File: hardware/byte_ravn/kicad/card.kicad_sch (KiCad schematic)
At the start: 13 parts, among them J3 Bus_Apple_II_Card_Side, U11 SN74LVC8T245, U12 SN74LVC8T245, U13 SN74LVC8T245, U14 SN74LVC8T245, U8 SN74LVC8T245, U9 SN74LVC8T245

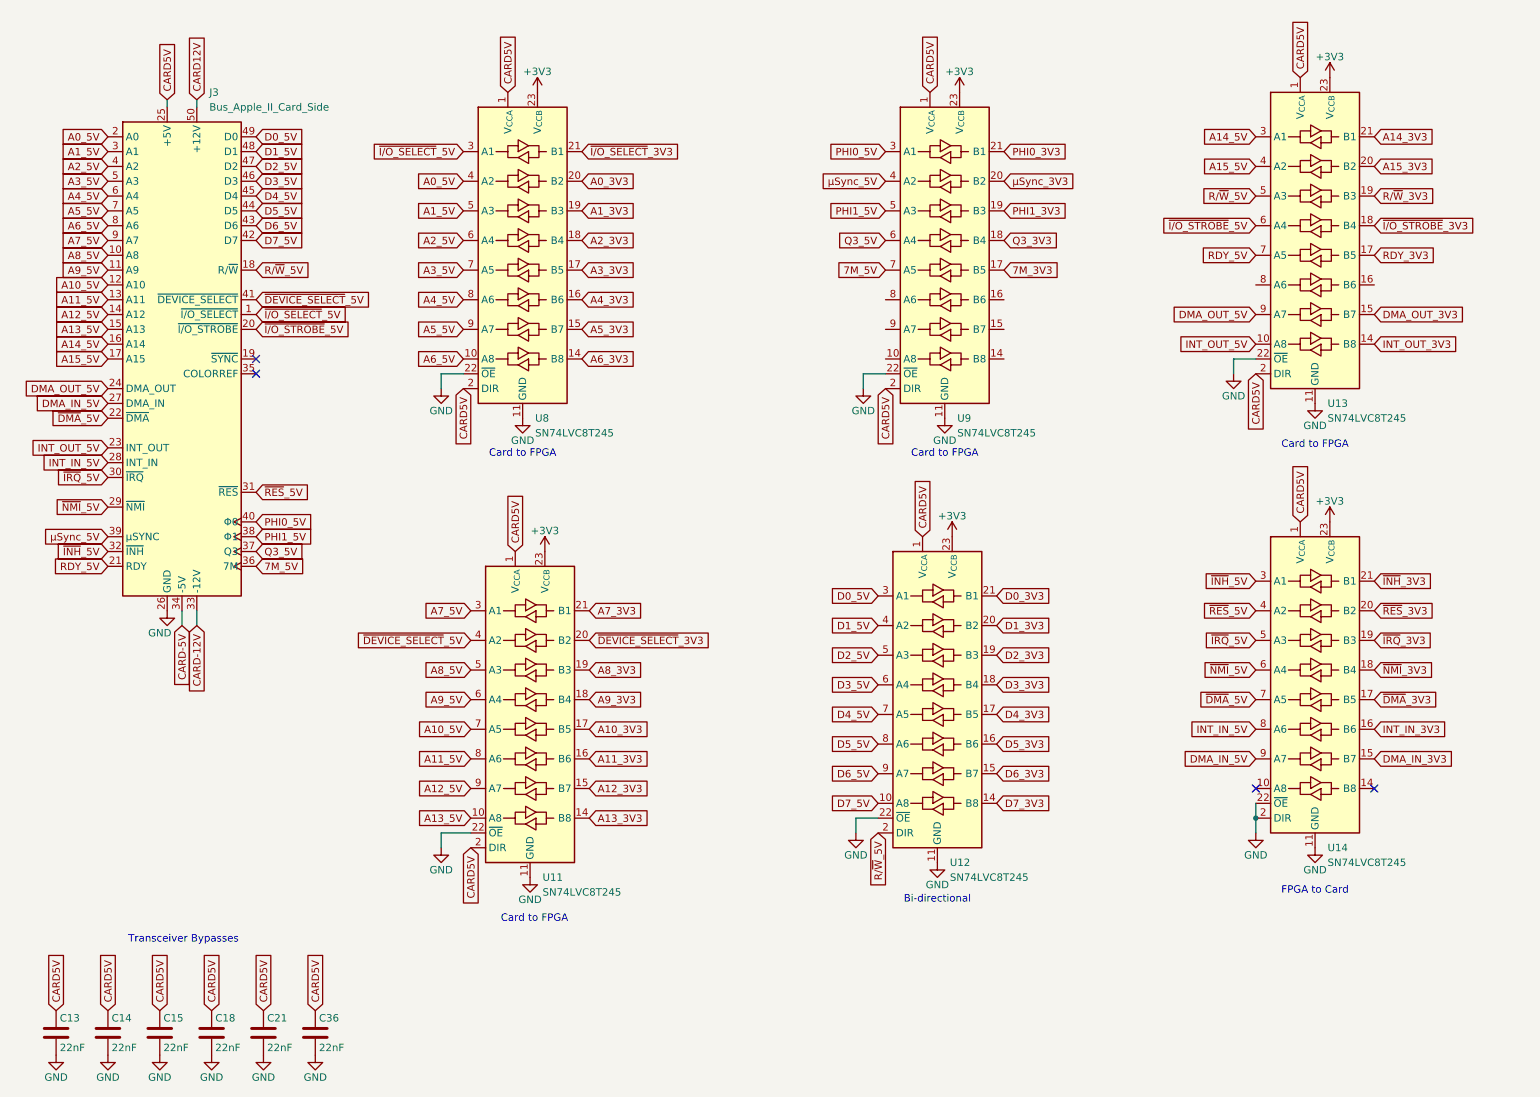
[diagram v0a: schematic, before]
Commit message: Updates to Ravn
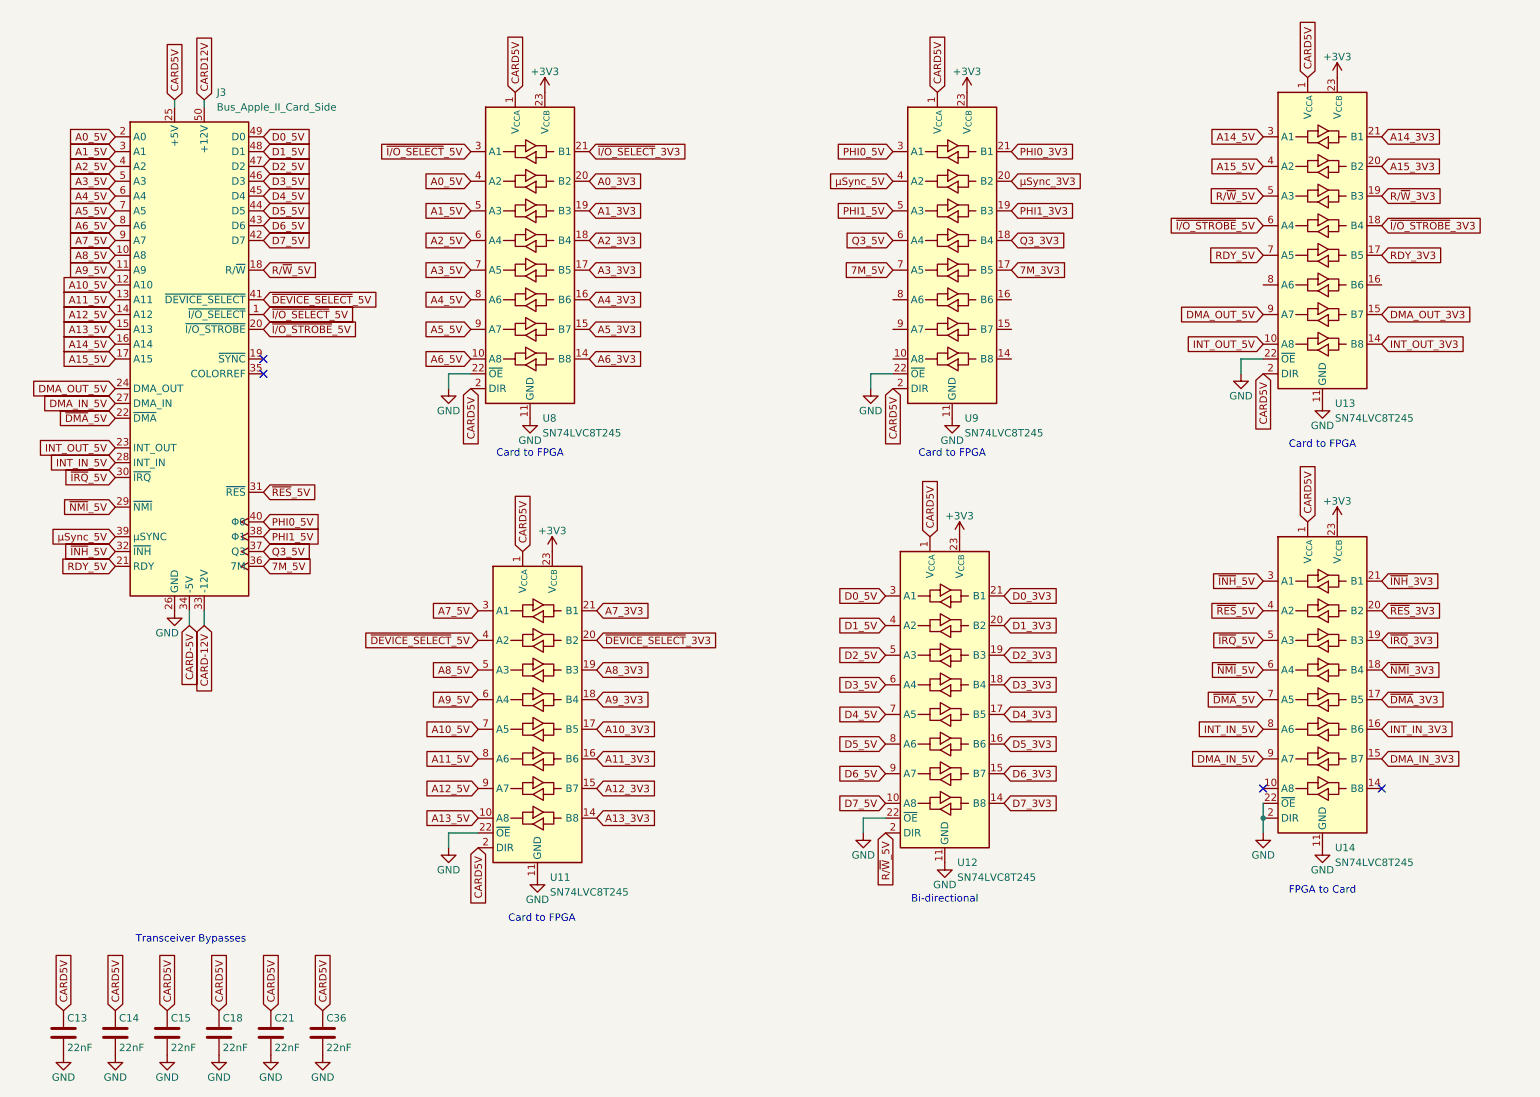
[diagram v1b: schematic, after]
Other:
- moved on the sheet: C13, C14, C15, C18, C21, C36, J3, U11, U12, U13, U14, U8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
